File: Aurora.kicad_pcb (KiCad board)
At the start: 2 copper layers, 57.1 x 62.7 mm, 58 parts, among them SW2 SW_Push, SW3 SW_SPDT, U1 IS31FL3736, U2 PRTR5V0U2X, U3 STM32F072CBUx, U4 MCP1700-3002E_SOT23

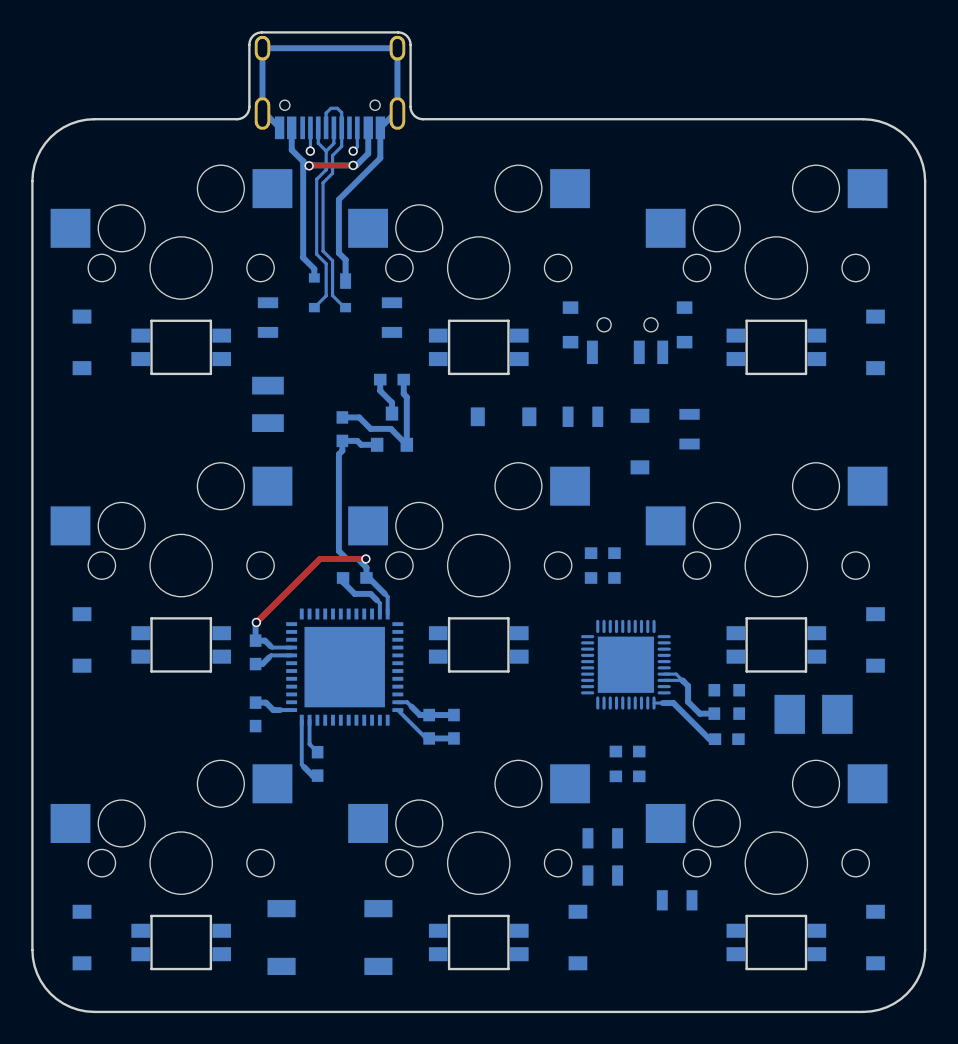
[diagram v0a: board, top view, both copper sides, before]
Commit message: Route it
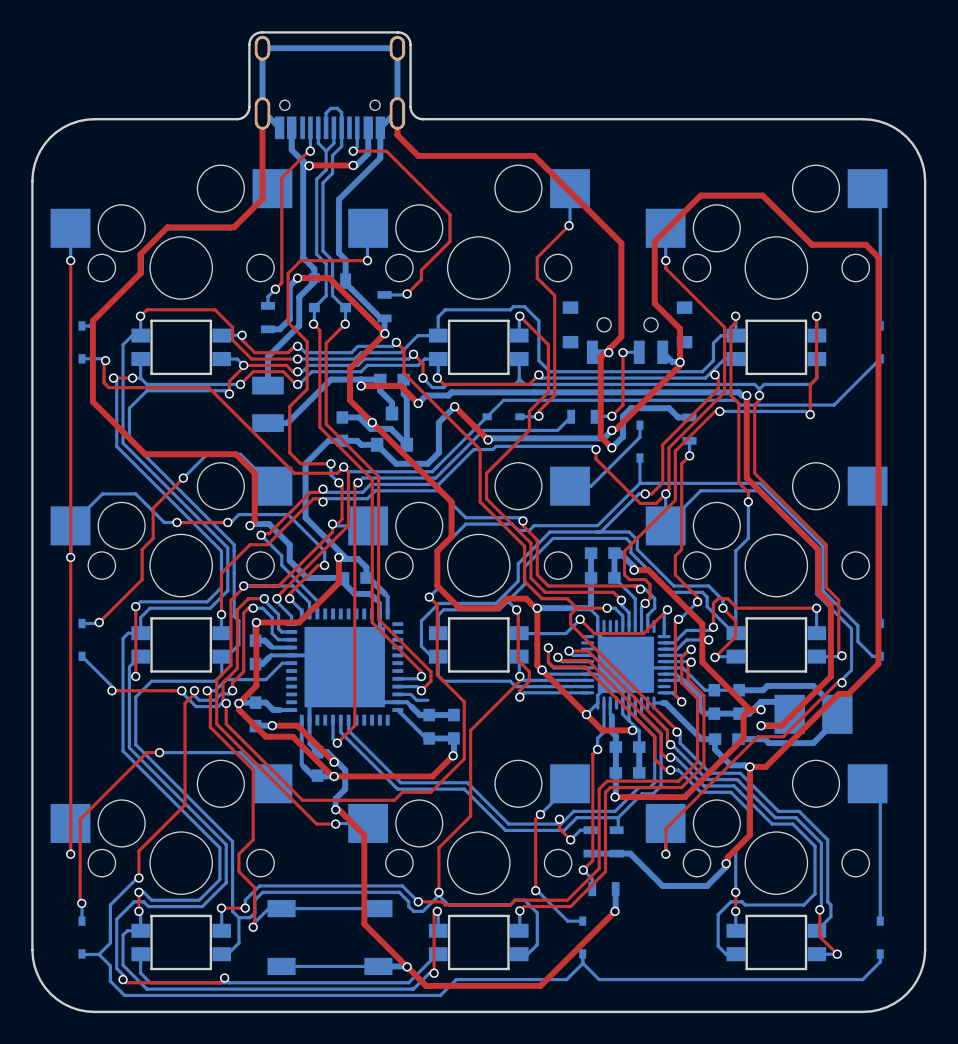
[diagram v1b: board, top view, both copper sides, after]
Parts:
- D1, D2, D3, D4, D5, D6, D7, D8, D9: footprint Diodes_SMD:D_SOD-123 -> Diodes_SMD:D_SOD-323
- R1, R2, R3, R4, R5, R73, R74: footprint Resistors_SMD:R_0805 -> Resistors_SMD:R_0603
- moved R1 4.74 mm to (66.8, 79.5), turned to 180 degrees
- moved R4 2.29 mm to (65.9, 76.4), turned to 270 degrees
- moved R3 0.92 mm to (67.6, 76.4), turned to 270 degrees
- moved R74 0.85 mm to (52.7, 42.2)
- moved D6 0.30 mm to (65.4, 82.5)
- moved D7 0.30 mm to (84.4, 44.5)
- moved D8 0.30 mm to (84.4, 63.5)
- moved D9 0.30 mm to (84.4, 82.5)
- moved C6 0.29 mm to (68.3, 70.4)
- moved C7 0.22 mm to (68.3, 72.0)
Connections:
- LED1 pad 1: Net-(LED1-Pad1) -> CS1
- LED1 pad 2: Net-(LED1-Pad2) -> SW2
- LED1 pad 3: Net-(LED1-Pad3) -> SW1
- LED1 pad 4: Net-(LED1-Pad4) -> SW3
- LED2 pad 1: Net-(LED2-Pad1) -> CS2
- LED2 pad 2: Net-(LED2-Pad2) -> SW2
- LED2 pad 3: Net-(LED2-Pad3) -> SW1
- LED2 pad 4: Net-(LED2-Pad4) -> SW3
- LED3 pad 1: Net-(LED3-Pad1) -> CS3
- LED3 pad 2: Net-(LED3-Pad2) -> SW2
- LED3 pad 3: Net-(LED3-Pad3) -> SW1
- LED3 pad 4: Net-(LED3-Pad4) -> SW3
- LED4 pad 1: Net-(LED4-Pad1) -> CS4
- LED4 pad 2: Net-(LED4-Pad2) -> SW2
- LED4 pad 3: Net-(LED4-Pad3) -> SW1
- LED4 pad 4: Net-(LED4-Pad4) -> SW3
- LED5 pad 1: Net-(LED5-Pad1) -> CS5
- LED5 pad 2: Net-(LED5-Pad2) -> SW2
- LED5 pad 3: Net-(LED5-Pad3) -> SW1
- LED5 pad 4: Net-(LED5-Pad4) -> SW3
- LED6 pad 1: Net-(LED6-Pad1) -> CS6
- LED6 pad 2: Net-(LED6-Pad2) -> SW2
- LED6 pad 3: Net-(LED6-Pad3) -> SW1
- LED6 pad 4: Net-(LED6-Pad4) -> SW3
- LED7 pad 1: Net-(LED7-Pad1) -> CS7
- LED7 pad 2: Net-(LED7-Pad2) -> SW2
- LED7 pad 3: Net-(LED7-Pad3) -> SW1
- LED7 pad 4: Net-(LED7-Pad4) -> SW3
- LED8 pad 1: Net-(LED8-Pad1) -> CS8
- LED8 pad 2: Net-(LED8-Pad2) -> SW2
- LED8 pad 3: Net-(LED8-Pad3) -> SW1
- LED8 pad 4: Net-(LED8-Pad4) -> SW3
- LED9 pad 1: Net-(LED9-Pad1) -> CS1
- LED9 pad 2: Net-(LED9-Pad2) -> SW5
- LED9 pad 3: Net-(LED9-Pad3) -> SW4
- LED9 pad 4: Net-(LED9-Pad4) -> SW6
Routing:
- net GND: track 52.8 -> 335.0 mm, vias 0 -> 15
- net SW1: track 0.00 -> 192.6 mm, vias 0 -> 10
- net SW2: track 0.00 -> 189.3 mm, vias 0 -> 14
- net SW3: track 0.00 -> 167.9 mm, vias 0 -> 9
- net +3V3: track 44.0 -> 181.0 mm, vias 2 -> 11
- net +5V: track 8.59 -> 118.6 mm, vias 0 -> 8
- net COL2: track 0.00 -> 99.9 mm, vias 0 -> 7
- net ROW1: track 0.00 -> 95.6 mm, vias 0 -> 5
- net ROW2: track 0.00 -> 88.7 mm, vias 0 -> 4
- net ROW0: track 0.00 -> 71.1 mm, vias 0 -> 3
- net CS1: track 0.00 -> 69.0 mm, vias 0 -> 5
- net COL0: track 0.00 -> 68.6 mm, vias 0 -> 7
- net COL1: track 0.00 -> 64.7 mm, vias 0 -> 6
- net CS7: track 0.00 -> 49.9 mm, vias 0 -> 4
- net CS4: track 0.00 -> 40.8 mm, vias 0 -> 4
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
